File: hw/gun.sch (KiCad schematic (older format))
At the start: 53 parts, among them J1 SWD_01X04, J2 IDC_02X05, SW1 FUSE, SW2 BANG, U1 OSRB38C9BA, U2 ULN2003, U3 ULN2003, U4 MCP1826S, U5 74AHC1G08, U6 STM32F042F6Px, U7 74AHC1G08, U8 MCP1826S, U9 74AHC1G08

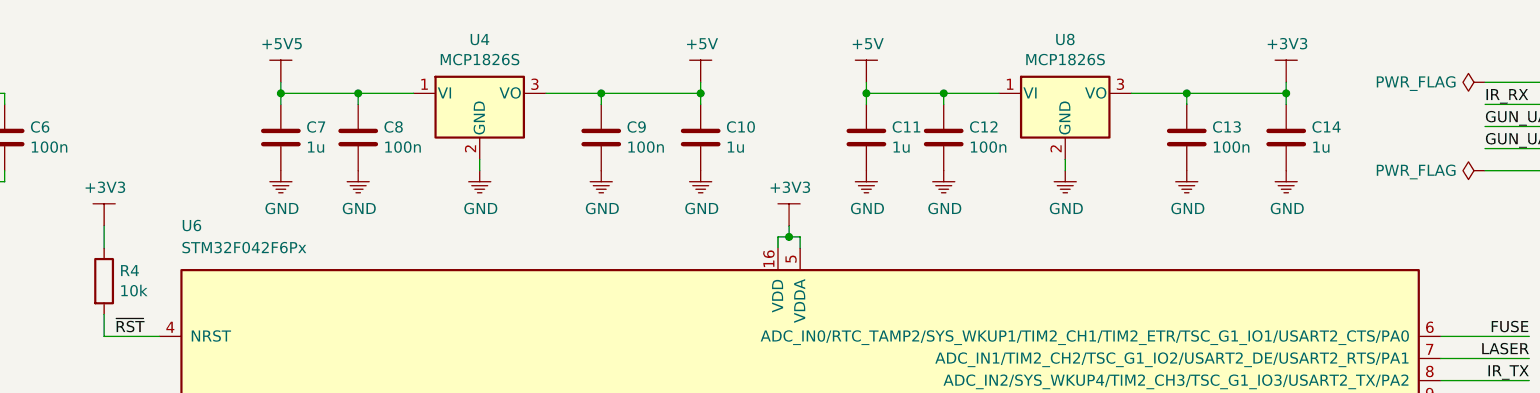
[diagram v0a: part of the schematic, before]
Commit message: updated schematic
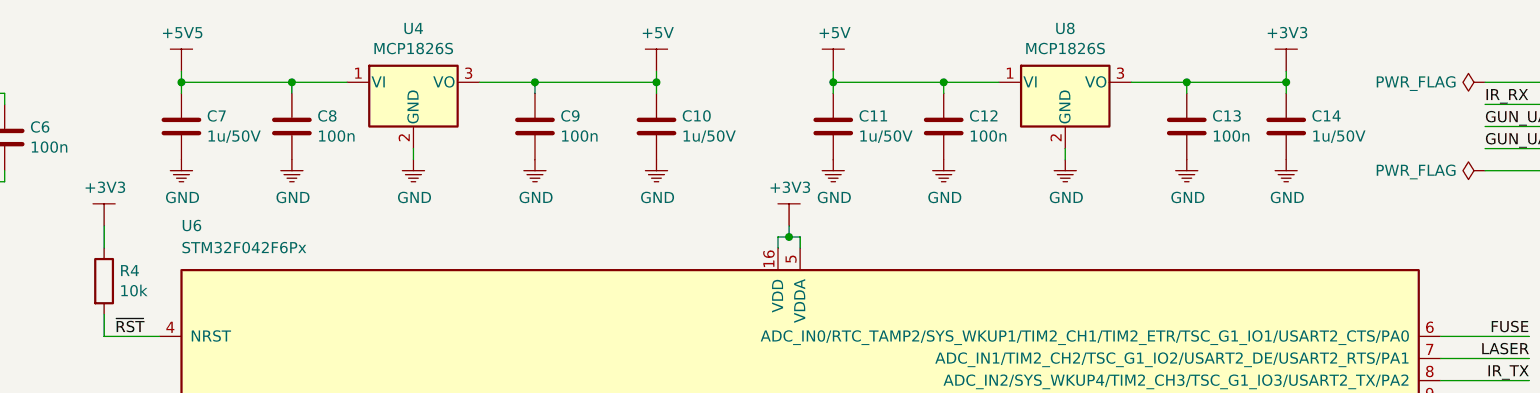
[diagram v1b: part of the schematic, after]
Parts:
- C1, C12, C13, C15, C16, C2, C3, C5, C6, C8, C9: footprint (none) -> Capacitor_SMD:C_0805_2012Metric
- C10, C11, C14, C7: value 1u -> 1u/50V; footprint (none) -> Capacitor_SMD:C_0805_2012Metric
- C4: footprint (none) -> Capacitor_Tantalum_SMD:CP_EIA-7343-31_Kemet-D
- D1, D2, D3, D4: footprint (none) -> Connector_PinHeader_2.54mm:PinHeader_1x02_P2.54mm_Vertical
- R1, R10, R11, R12, R13, R14, R4, R7, R8, R9: footprint (none) -> Resistor_SMD:R_0805_2012Metric
- R2, R3, R5, R6: footprint (none) -> Resistor_SMD:R_1210_3225Metric
- SW1, SW2: footprint (none) -> Connector_PinHeader_2.54mm:PinHeader_2x01_P2.54mm_Vertical
- U2, U3: footprint (none) -> Package_SO:SOIC-16_3.9x9.9mm_P1.27mm
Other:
- moved on the sheet: C10, C11, C12, C13, C14, C7, C8, C9, U4, U8
